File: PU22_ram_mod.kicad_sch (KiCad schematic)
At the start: 7 parts, among them J1 MOBO, J2 BA8, J3 BA10

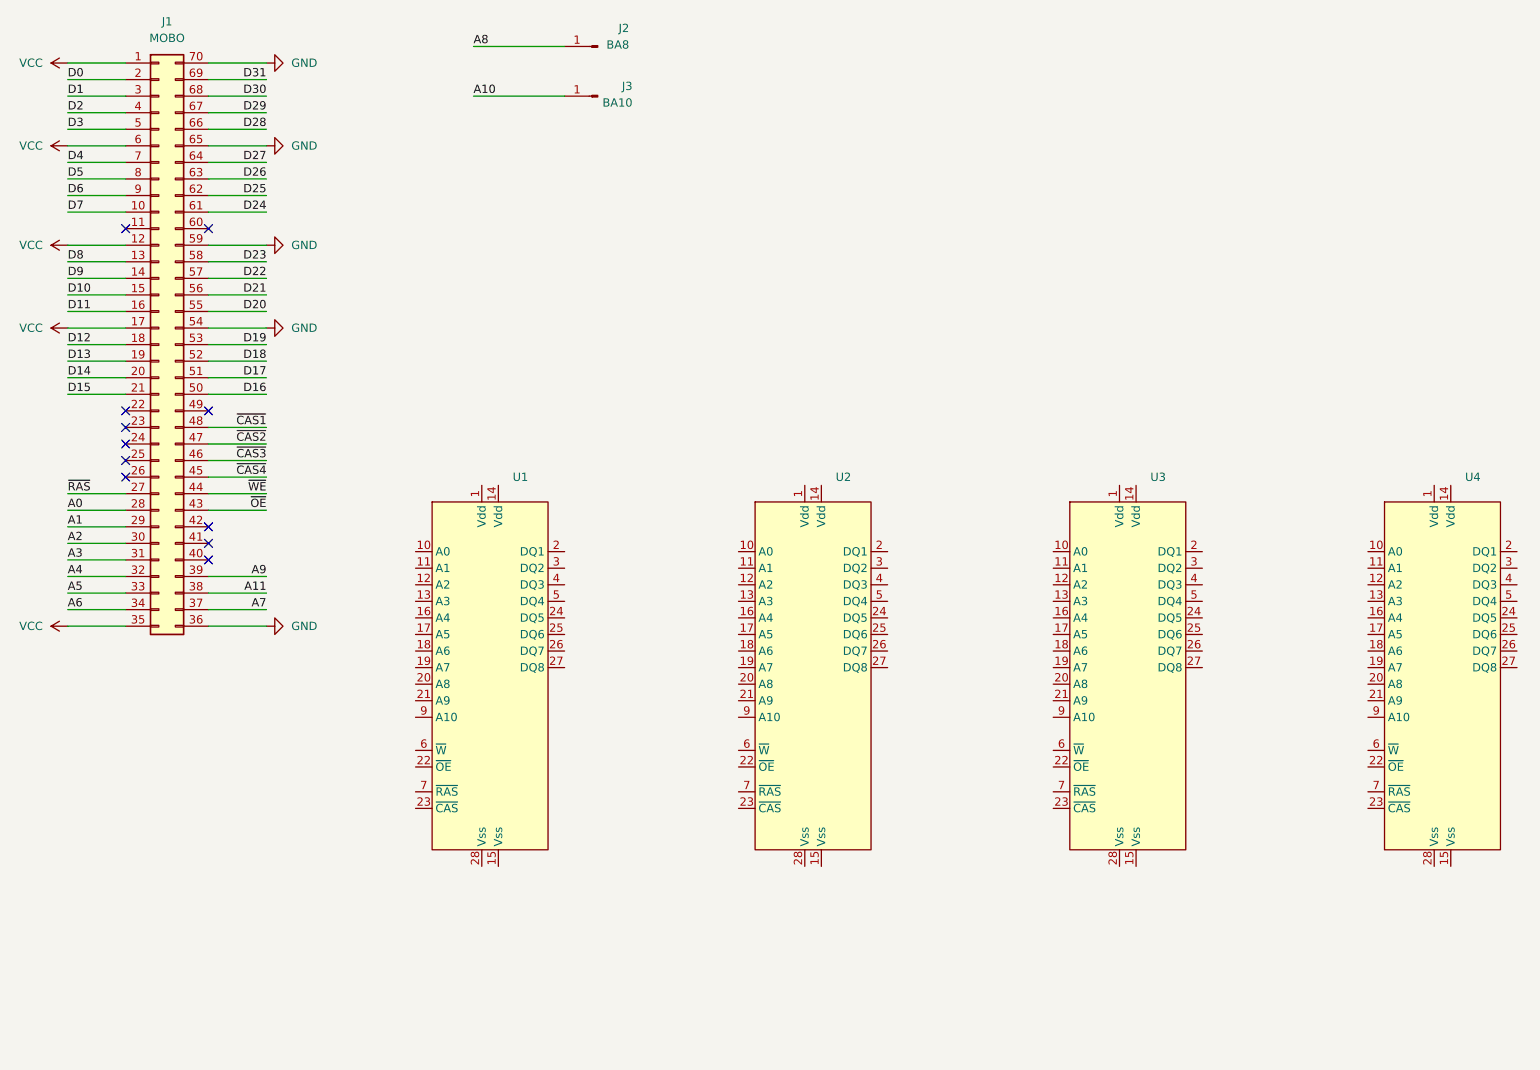
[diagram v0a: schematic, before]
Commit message: Update schematic
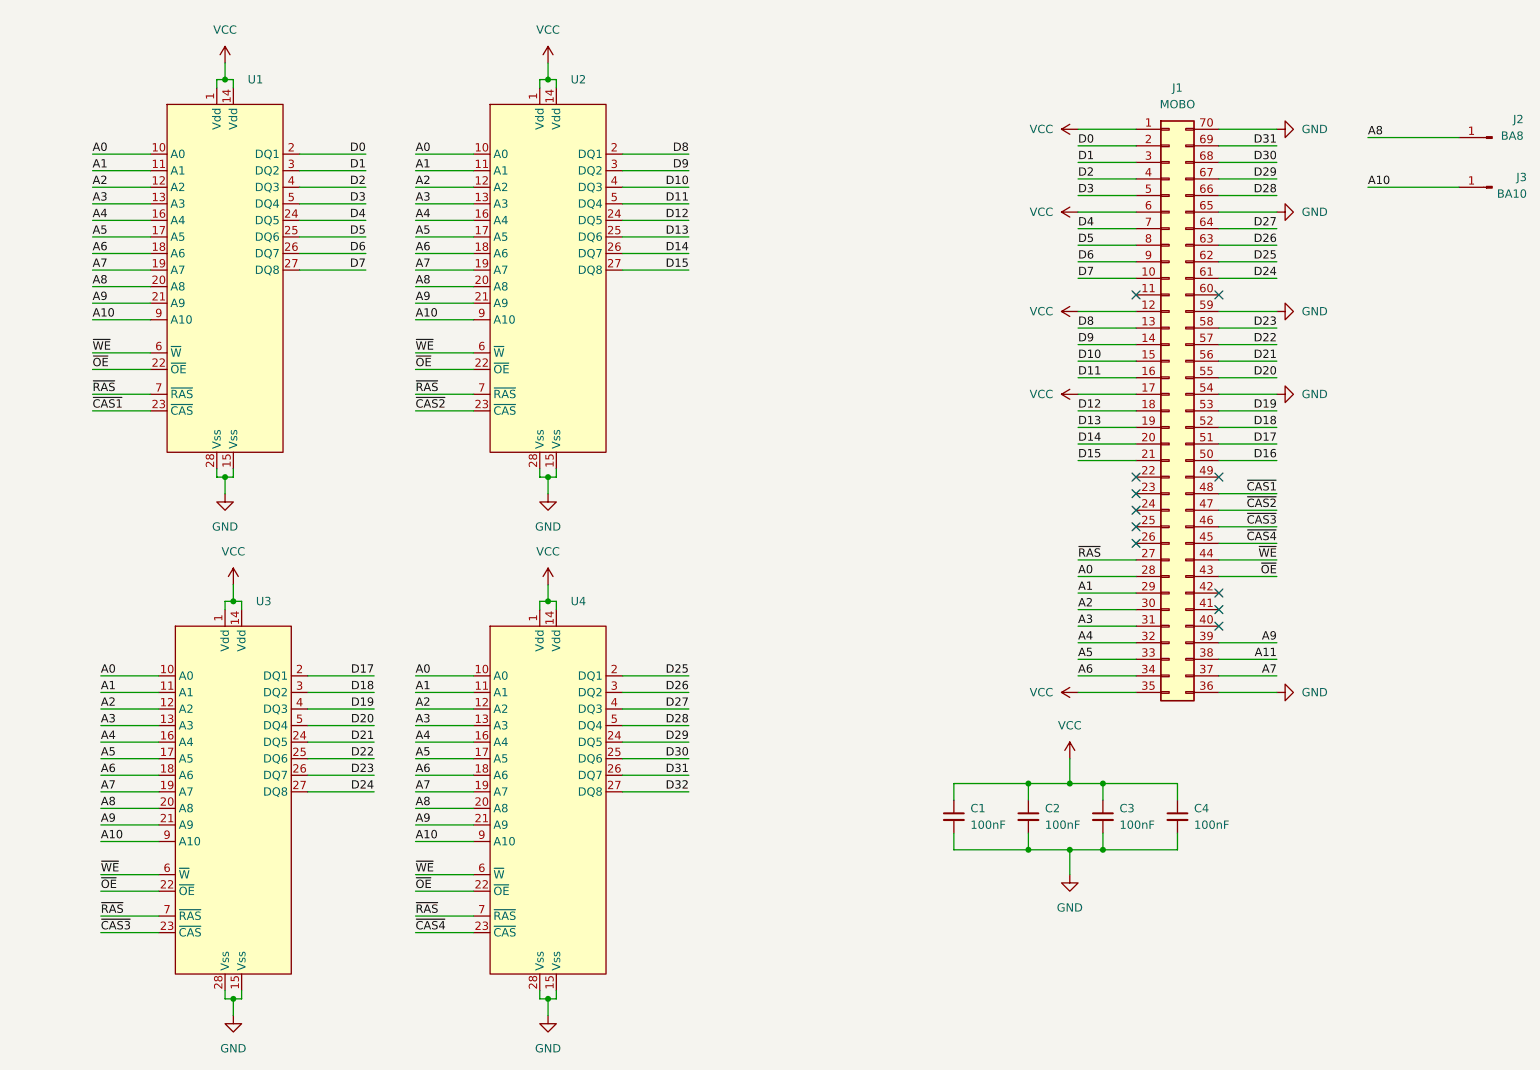
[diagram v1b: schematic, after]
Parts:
- added C1, C2, C3, C4: 100nF, Capacitor_SMD:C_1206_3216Metric_Pad1.33x1.80mm_HandSolder, symbol Device:C_Small
- J2, J3: footprint TestPoint:TestPoint_Pad_D4.0mm -> TestPoint:TestPoint_Pad_D2.5mm
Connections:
- net A0: now also U1.10 (A0), U2.10 (A0), U3.10 (A0), U4.10 (A0)
- net A1: now also U1.11 (A1), U2.11 (A1), U3.11 (A1), U4.11 (A1)
- net A10: now also U1.9 (A10), U2.9 (A10), U3.9 (A10), U4.9 (A10)
- net A2: now also U1.12 (A2), U2.12 (A2), U3.12 (A2), U4.12 (A2)
- net A3: now also U1.13 (A3), U2.13 (A3), U3.13 (A3), U4.13 (A3)
- net A4: now also U1.16 (A4), U2.16 (A4), U3.16 (A4), U4.16 (A4)
- net A5: now also U1.17 (A5), U2.17 (A5), U3.17 (A5), U4.17 (A5)
- net A6: now also U1.18 (A6), U2.18 (A6), U3.18 (A6), U4.18 (A6)
- net A7: now also U1.19 (A7), U2.19 (A7), U3.19 (A7), U4.19 (A7)
- net A8: now also U1.20 (A8), U2.20 (A8), U3.20 (A8), U4.20 (A8)
- net A9: now also U1.21 (A9), U2.21 (A9), U3.21 (A9), U4.21 (A9)
- net D0: now also U1.2 (DQ1)
- net D1: now also U1.3 (DQ2)
- net D10: now also U2.4 (DQ3)
- net D11: now also U2.5 (DQ4)
- net D12: now also U2.24 (DQ5)
- net D13: now also U2.25 (DQ6)
- net D14: now also U2.26 (DQ7)
- net D15: now also U2.27 (DQ8)
- net D17: now also U3.2 (DQ1)
- net D18: now also U3.3 (DQ2)
- net D19: now also U3.4 (DQ3)
- net D2: now also U1.4 (DQ3)
- net D20: now also U3.5 (DQ4)
- net D21: now also U3.24 (DQ5)
- net D22: now also U3.25 (DQ6)
- net D23: now also U3.26 (DQ7)
- net D24: now also U3.27 (DQ8)
- net D25: now also U4.2 (DQ1)
- net D26: now also U4.3 (DQ2)
- net D27: now also U4.4 (DQ3)
- net D28: now also U4.5 (DQ4)
- net D29: now also U4.24 (DQ5)
- net D3: now also U1.5 (DQ4)
- net D30: now also U4.25 (DQ6)
- net D31: now also U4.26 (DQ7)
- net D4: now also U1.24 (DQ5)
- net D5: now also U1.25 (DQ6)
- net D6: now also U1.26 (DQ7)
- net D7: now also U1.27 (DQ8)
- net D8: now also U2.2 (DQ1)
- net D9: now also U2.3 (DQ2)
- net GND: now also U1.15 (Vss), U1.28 (Vss), U2.15 (Vss), U2.28 (Vss), U3.15 (Vss), U3.28 (Vss), U4.15 (Vss), U4.28 (Vss), C1.2, C2.2, C3.2, C4.2
- net VCC: now also U1.1 (Vdd), U1.14 (Vdd), U2.1 (Vdd), U2.14 (Vdd), U3.1 (Vdd), U3.14 (Vdd), U4.1 (Vdd), U4.14 (Vdd), C1.1, C2.1, C3.1, C4.1
- net ~{CAS1}: now also U1.23 (~{CAS})
- net ~{CAS2}: now also U2.23 (~{CAS})
- net ~{CAS3}: now also U3.23 (~{CAS})
- net ~{CAS4}: now also U4.23 (~{CAS})
- net ~{OE}: now also U1.22 (~{OE}), U2.22 (~{OE}), U3.22 (~{OE}), U4.22 (~{OE})
- net ~{RAS}: now also U1.7 (~{RAS}), U2.7 (~{RAS}), U3.7 (~{RAS}), U4.7 (~{RAS})
- net ~{WE}: now also U1.6 (~{W}), U2.6 (~{W}), U3.6 (~{W}), U4.6 (~{W})
- net D32: now reaches U4.27 (DQ8)
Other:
- moved on the sheet: J1, J2, J3, U1, U2, U3, U4
